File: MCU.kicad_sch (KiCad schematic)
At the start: 43 parts, among them J1 Micro_SD_Card, J1 SM03B-SRSS-TB

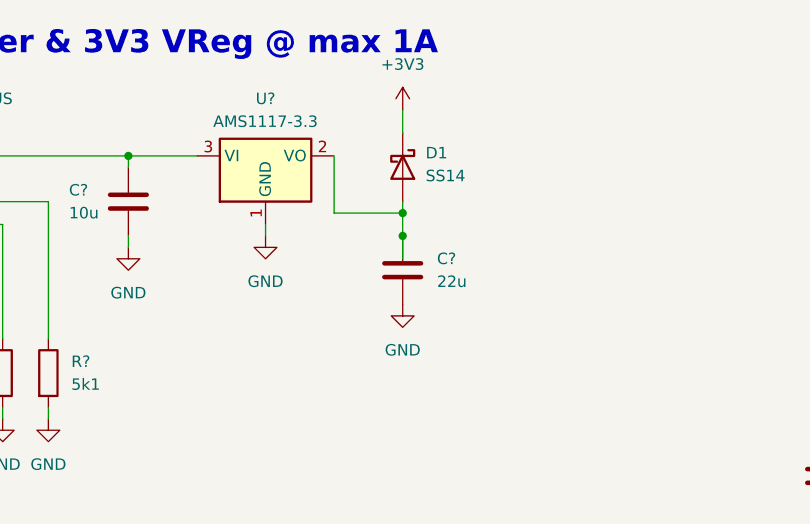
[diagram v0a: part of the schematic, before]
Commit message: mcu
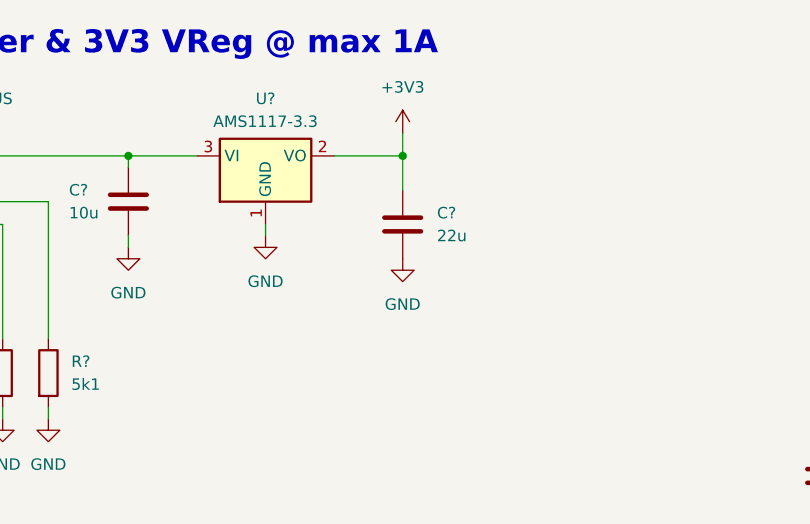
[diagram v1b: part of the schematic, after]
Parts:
- removed D1: SS14, Diode_SMD:D_SMA, symbol Diode:SS14
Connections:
- net +3V3: now also C?.1, U?.2 (VO)
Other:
- moved on the sheet: C?
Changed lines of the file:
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@@
 	)
 	(junction
+		(at 106.68 29.21)
+		(diameter 0)
+		(color 0 0 0 0)
+	)
+	(junction
 		(at 228.6 80.01)
 		(diameter 0)
@@
 	)
 	(junction
-		(at 106.68 35.56)
-		(diameter 0)
-		(color 0 0 0 0)
-	)
-	(junction
 		(at 40.64 175.26)
 		(diameter 0)
@@
 	)
 	(junction
-		(at 106.68 38.1)
-		(diameter 0)
-		(color 0 0 0 0)
-	)
-	(junction
 		(at 287.02 59.69)
 		(diameter 0)
@@
 	(wire
 		(pts
-			(xy 106.68 40.64) (xy 106.68 38.1)
+			(xy 106.68 29.21) (xy 106.68 33.02)
 		)
 		(stroke
@@
 	(wire
 		(pts
+			(xy 99.06 29.21) (xy 106.68 29.21)
+		)
+		(stroke
+			(width 0)
+			(type default)
+		)
+	)
+	(wire
+		(pts
 			(xy 144.78 128.27) (xy 144.78 130.81)
 		)
@@
 	(wire
 		(pts
-			(xy 99.06 35.56) (xy 99.06 29.21)
-		)
-		(stroke
-			(width 0)
-			(type default)
-		)
-	)
-	(wire
-		(pts
 			(xy 255.27 196.85) (xy 255.27 199.39)
 		)
@@
 	(wire
 		(pts
-			(xy 106.68 24.13) (xy 106.68 26.67)
+			(xy 106.68 26.67) (xy 106.68 29.21)
 		)
 		(stroke
@@
 	(wire
 		(pts
-			(xy 99.06 35.56) (xy 106.68 35.56)
-		)
-		(stroke
-			(width 0)
-			(type default)
-		)
-	)
-	(wire
-		(pts
 			(xy 213.36 80.01) (xy 215.9 80.01)
 		)
@@
 	(wire
 		(pts
-			(xy 106.68 38.1) (xy 106.68 35.56)
-		)
-		(stroke
-			(width 0)
-			(type default)
-		)
-	)
-	(wire
-		(pts
 			(xy 163.83 128.27) (xy 180.34 128.27)
 		)
@@
 	(wire
 		(pts
-			(xy 106.68 34.29) (xy 106.68 35.56)
-		)
-		(stroke
-			(width 0)
-			(type default)
-		)
-	)
-	(wire
-		(pts
 			(xy 236.22 69.85) (xy 248.92 69.85)
 		)
@@
 	(symbol
 		(lib_id "power:GND")
-		(at 106.68 45.72 0)
+		(at 106.68 40.64 0)
 		(unit 1)
 		(exclude_from_sim no)
@@
 		(fields_autoplaced yes)
 		(property "Reference" "#PWR?"
-			(at 106.68 52.07 0)
+			(at 106.68 46.99 0)
 			(effects
 				(font
@@
 		)
 		(property "Value" "GND"
-			(at 106.68 50.8 0)
+			(at 106.68 45.72 0)
 			(effects
 				(font
@@
 		)
 		(property "Footprint" ""
-			(at 106.68 45.72 0)
+			(at 106.68 40.64 0)
 			(effects
 				(font
@@
 		)
 		(property "Datasheet" ""
-			(at 106.68 45.72 0)
+			(at 106.68 40.64 0)
 			(effects
 				(font
@@
 		)
 		(property "Description" "Power symbol creates a global label with name \"GND\" , ground"
-			(at 106.68 45.72 0)
+			(at 106.68 40.64 0)
 			(effects
 				(font
@@
 	(symbol
 		(lib_id "power:+3V3")
-		(at 106.68 24.13 0)
+		(at 106.68 26.67 0)
 		(unit 1)
 		(exclude_from_sim no)
@@
 		(fields_autoplaced yes)
 		(property "Reference" "#PWR?"
-			(at 106.68 27.94 0)
+			(at 106.68 30.48 0)
 			(effects
 				(font
@@
 		)
 		(property "Value" "+3V3"
-			(at 106.68 19.05 0)
+			(at 106.68 21.59 0)
 			(effects
 				(font
@@
 		)
 		(property "Footprint" ""
-			(at 106.68 24.13 0)
+			(at 106.68 26.67 0)
 			(effects
 				(font
@@
 		)
 		(property "Datasheet" ""
-			(at 106.68 24.13 0)
+			(at 106.68 26.67 0)
 			(effects
 				(font
@@
 		)
 		(property "Description" "Power symbol creates a global label with name \"+3V3\""
-			(at 106.68 24.13 0)
+			(at 106.68 26.67 0)
 			(effects
 				(font
@@
 	)
 	(symbol
-		(lib_id "Diode:SS14")
-		(at 106.68 30.48 270)
-		(unit 1)
-		(exclude_from_sim no)
-		(in_bom yes)
-		(on_board yes)
-		(dnp no)
-		(fields_autoplaced yes)
-		(property "Reference" "D1"
-			(at 109.22 28.8924 90)
-			(effects
-				(font
-					(size 1.27 1.27)
-				)
-				(justify left)
-			)
-		)
-		(property "Value" "SS14"
-			(at 109.22 31.4324 90)
-			(effects
-				(font
-					(size 1.27 1.27)
-				)
-				(justify left)
-			)
-		)
-		(property "Footprint" "Diode_SMD:D_SMA"
-			(at 102.235 30.48 0)
-			(effects
-				(font
-					(size 1.27 1.27)
-				)
-				(hide yes)
-			)
-		)
-		(property "Datasheet" "https://www.vishay.com/docs/88746/ss12.pdf"
-			(at 106.68 30.48 0)
-			(effects
-				(font
-					(size 1.27 1.27)
-				)
-				(hide yes)
-			)
-		)
-		(property "Description" "40V 1A Schottky Diode, SMA"
-			(at 106.68 30.48 0)
-			(effects
-				(font
-					(size 1.27 1.27)
-				)
-				(hide yes)
-			)
-		)
-		(pin "1"
-		)
-		(pin "2"
-		)
-		(instances
-			(project "MCU"
-				(path "/f6b69531-d30c-486d-b9b8-67bb2790b07b"
-					(reference "D1")
-					(unit 1)
-				)
-			)
-		)
-	)
-	(symbol
 		(lib_id "power:GND")
 		(at 124.46 123.19 0)
@@
 	(symbol
 		(lib_id "Device:C")
-		(at 106.68 41.91 0)
+		(at 106.68 36.83 0)
 		(unit 1)
 		(exclude_from_sim no)
@@
 		(fields_autoplaced yes)
 		(property "Reference" "C?"
-			(at 110.49 40.6399 0)
+			(at 110.49 35.5599 0)
 			(effects
 				(font
@@
 		)
 		(property "Value" "22u"
-			(at 110.49 43.1799 0)
+			(at 110.49 38.0999 0)
 			(effects
 				(font
@@
 		)
 		(property "Footprint" ""
-			(at 107.6452 45.72 0)
+			(at 107.6452 40.64 0)
 			(effects
 				(font
@@
 		)
 		(property "Datasheet" "~"
-			(at 106.68 41.91 0)
+			(at 106.68 36.83 0)
 			(effects
 				(font
@@
 		)
 		(property "Description" "Unpolarized capacitor"
-			(at 106.68 41.91 0)
+			(at 106.68 36.83 0)
 			(effects
 				(font
